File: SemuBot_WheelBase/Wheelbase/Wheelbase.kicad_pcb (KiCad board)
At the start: 2 copper layers, 84 x 65 mm, 83 parts, among them IC1 NCP164CSN330T1G, J1 10155435-00011LF, J10 B5B-XH-A_LF__SN_, J11 B5B-XH-A_LF__SN_, J12 B5B-XH-A_LF__SN_, J2 ftsh-105-01-l-dv-k, J3 TB003-500-P02BE, J4 B5B-XH-A_LF__SN_, J5 B5B-XH-A_LF__SN_, J6 B5B-XH-A_LF__SN_, J7 1984620, J8 1984620, J9 1984620, Q1 DI025N06PT-AQ, Q10 DI025N06PT-AQ, Q11 DI025N06PT-AQ, Q12 DI025N06PT-AQ, Q13 DI025N06PT-AQ, Q14 DI025N06PT-AQ, Q15 DI025N06PT-AQ, Q16 DI025N06PT-AQ, Q17 DI025N06PT-AQ, Q18 DI025N06PT-AQ, Q2 DI025N06PT-AQ, Q3 DI025N06PT-AQ, Q4 DI025N06PT-AQ, Q5 DI025N06PT-AQ, Q6 DI025N06PT-AQ, Q7 DI025N06PT-AQ, Q8 DI025N06PT-AQ, Q9 DI025N06PT-AQ, U1 STM32F303RET6, U2 DRV8353FSRTAR, U3 DRV8353FSRTAR, U4 DRV8353FSRTAR, Y1 WE-SPXO_CFPS-39

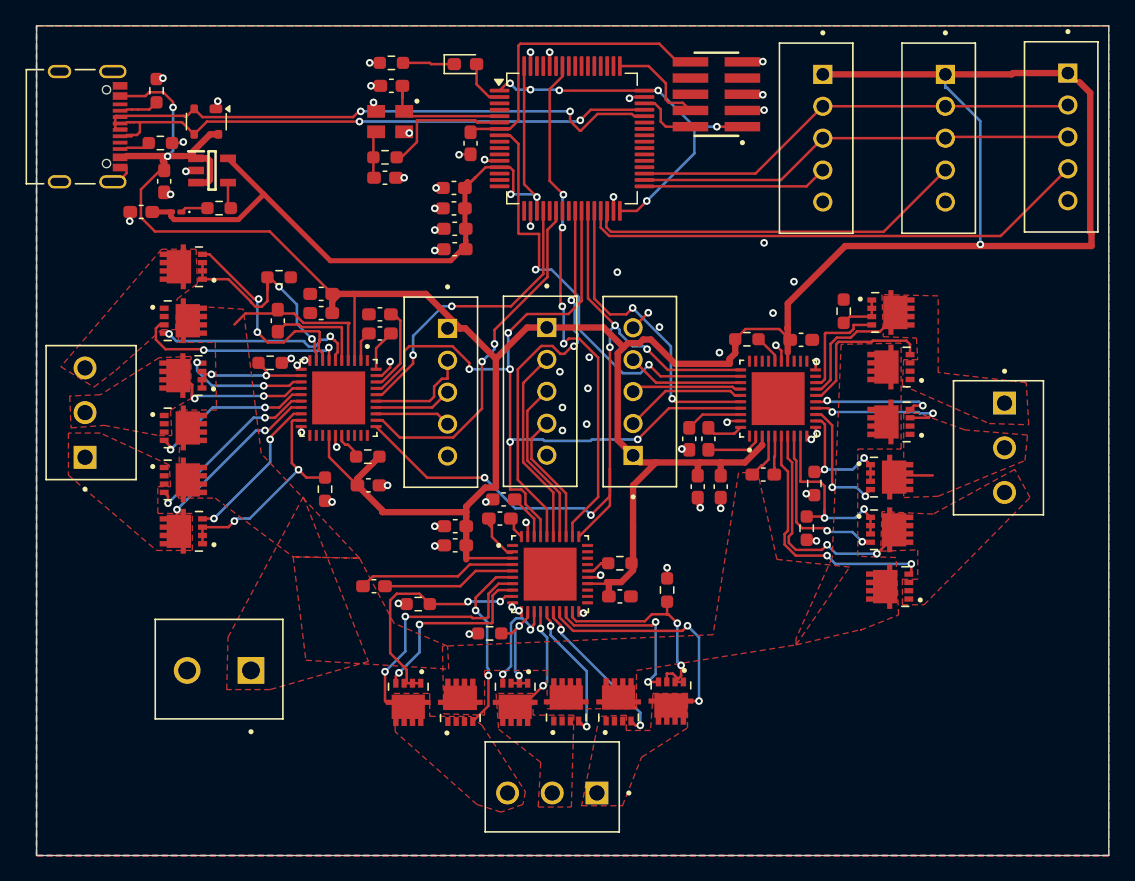
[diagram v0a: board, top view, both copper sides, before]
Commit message: Snapshot
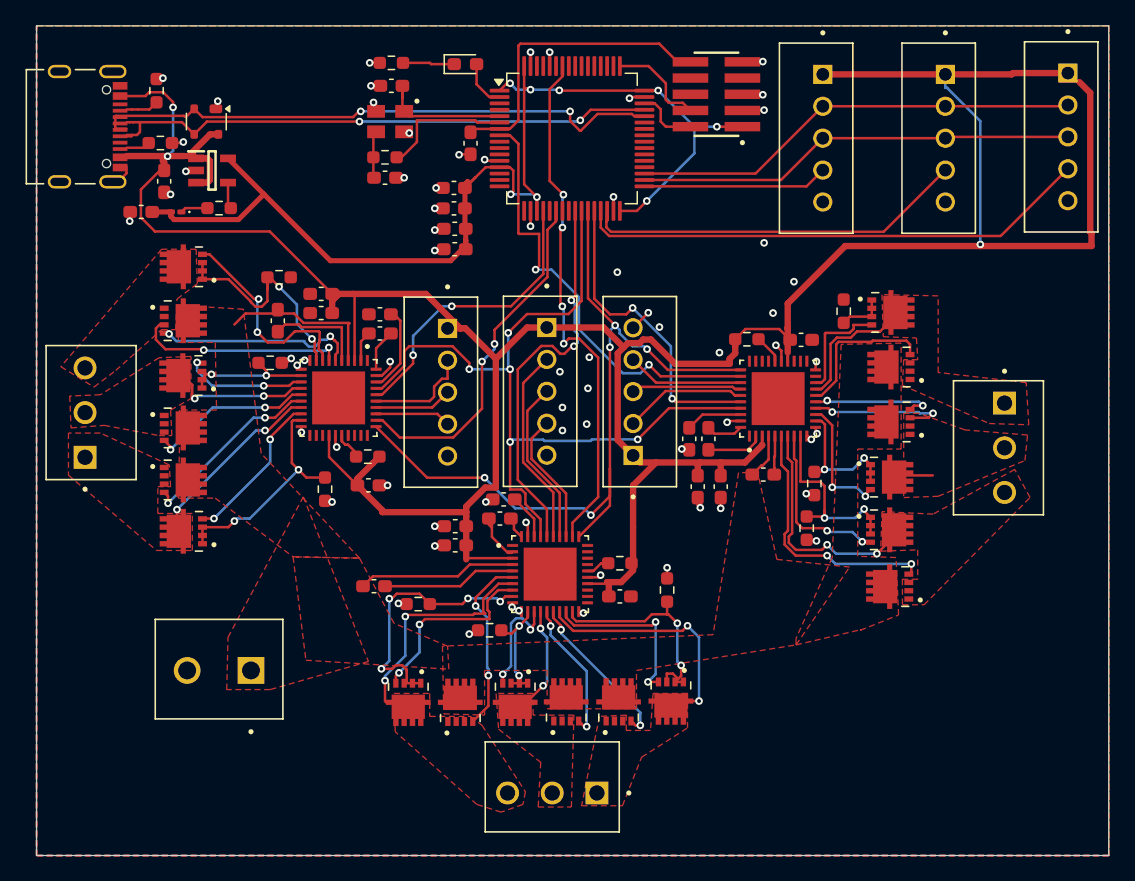
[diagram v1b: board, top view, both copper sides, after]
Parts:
- moved R17 0.25 mm to (148.2, 113.1)
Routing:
- net /Motor_3/SPA: track 18.8 -> 21.1 mm, vias 2 -> 4
